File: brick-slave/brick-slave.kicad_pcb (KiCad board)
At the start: 2 copper layers, 52.3 x 72.4 mm, 4 parts, among them J1 Conn_01x06_Male, J2 Conn_01x06_Male, J3 Conn_01x06_Female, J4 Conn_01x06_Female

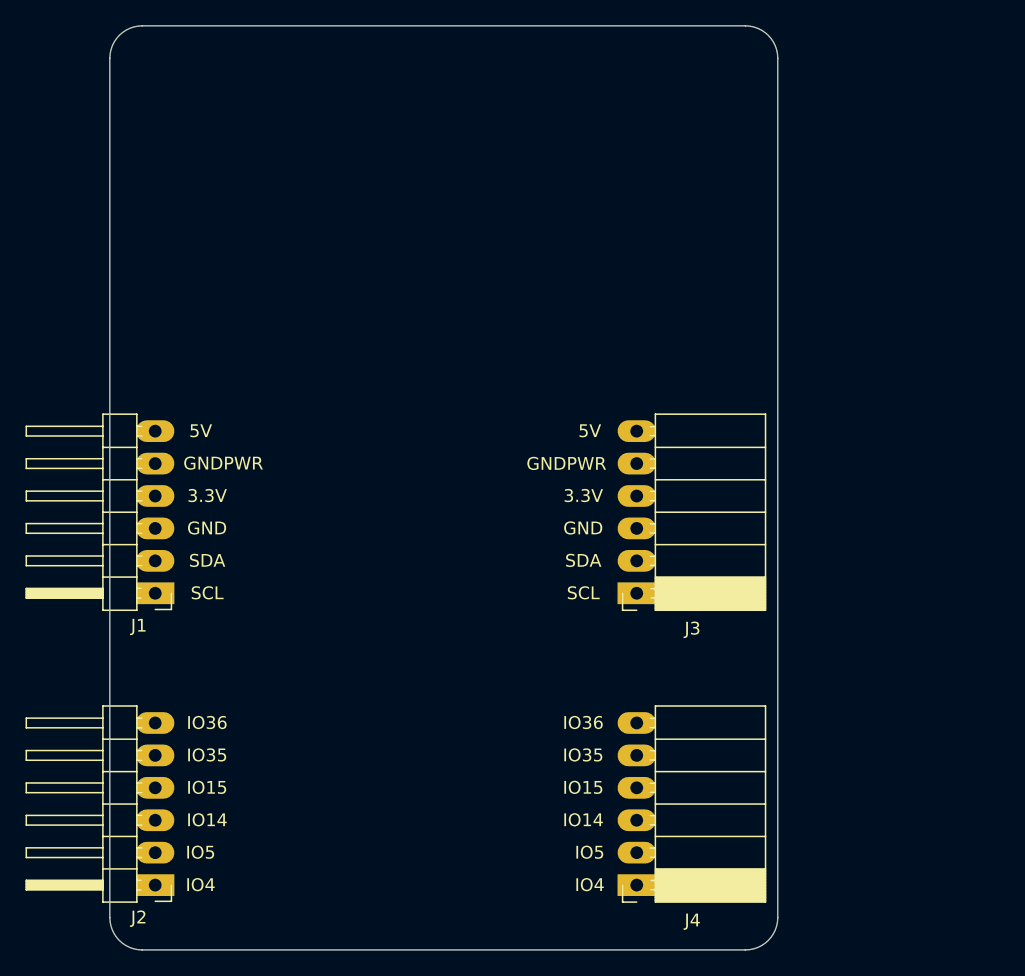
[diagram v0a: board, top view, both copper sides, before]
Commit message: refactor brick-slave
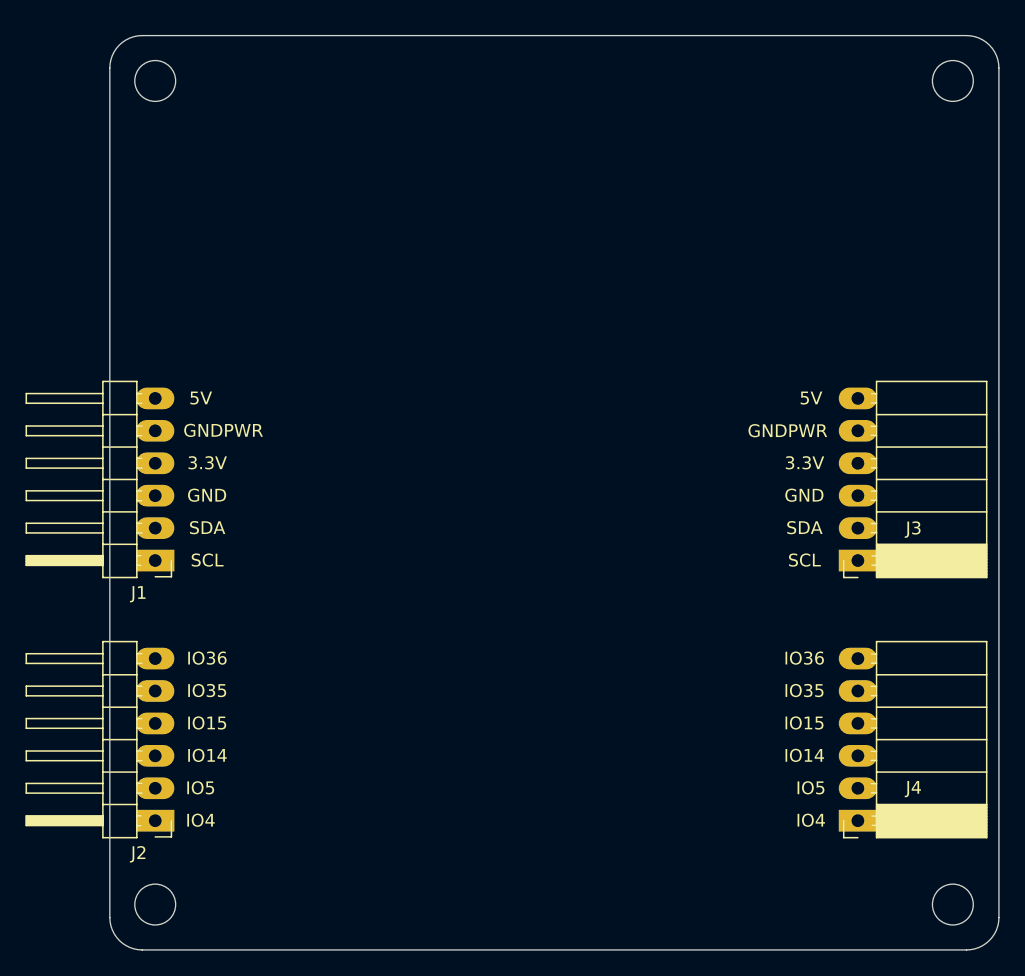
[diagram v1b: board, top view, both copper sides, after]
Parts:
- added H1: MountingHole, MountingHole:MountingHole_3.2mm_M3, F.Cu at (67.1, 58.9)
- added H2: MountingHole, MountingHole:MountingHole_3.2mm_M3, F.Cu at (129.5, 58.9)
- added H3: MountingHole, MountingHole:MountingHole_3.2mm_M3, F.Cu at (67.1, 123.4)
- added H4: MountingHole, MountingHole:MountingHole_3.2mm_M3, F.Cu at (129.5, 123.4)
- moved J4 18.0 mm to (122.1, 116.9)
- moved J3 17.5 mm to (122.1, 96.5)
- moved J2 5.05 mm to (67.1, 116.9)
- moved J1 2.56 mm to (67.1, 96.5)
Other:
- board size 52.3 x 72.4 mm -> 69.6 x 71.6 mm
